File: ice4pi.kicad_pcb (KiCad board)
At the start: 4 copper layers, 65 x 30 mm, 66 parts, among them J1 Pmod 2x6, J2 Raspberry_Pi_2_3, U1 ICE40HX1K-TQ144, U2 N25Q032A13ESC40F, U3 LT3030, U4 DSC1001DI1-012.0000, U5 TFDU4101-TR3

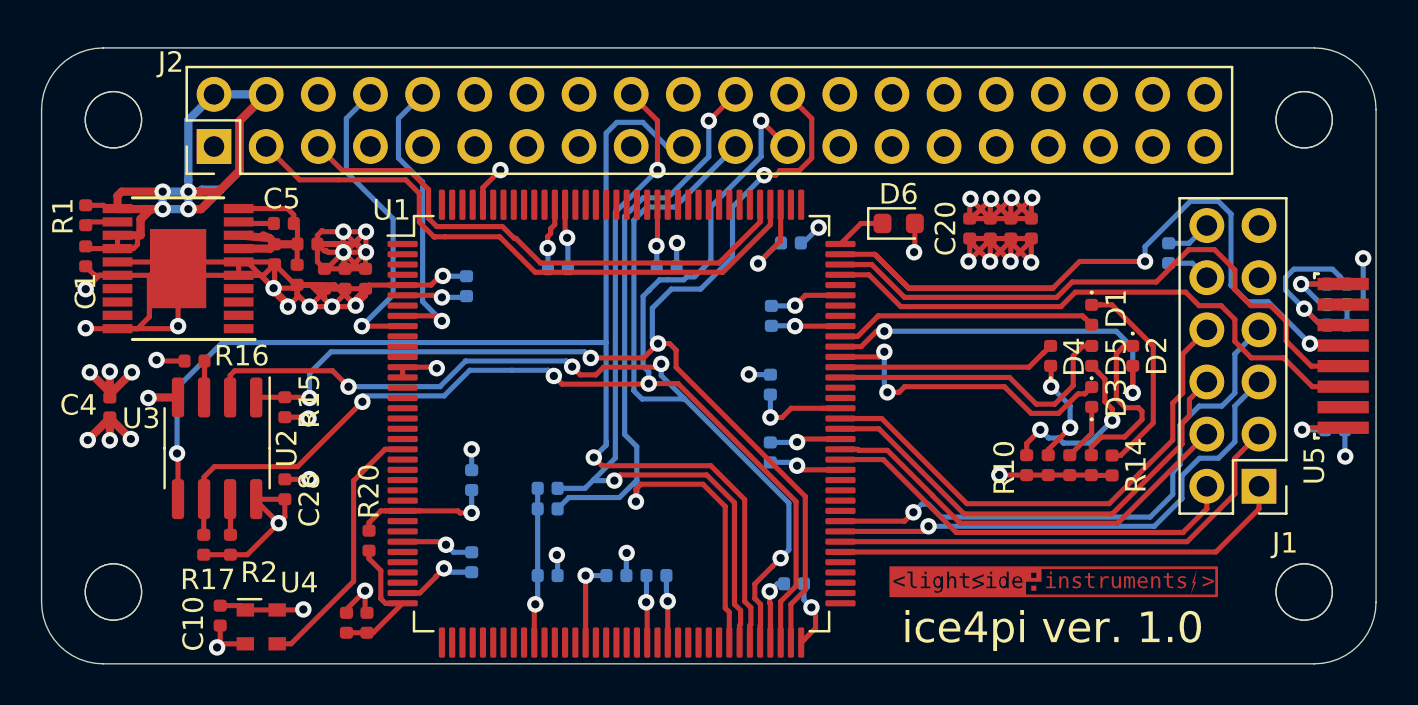
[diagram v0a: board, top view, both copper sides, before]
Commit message: Release ice4pi-1.1
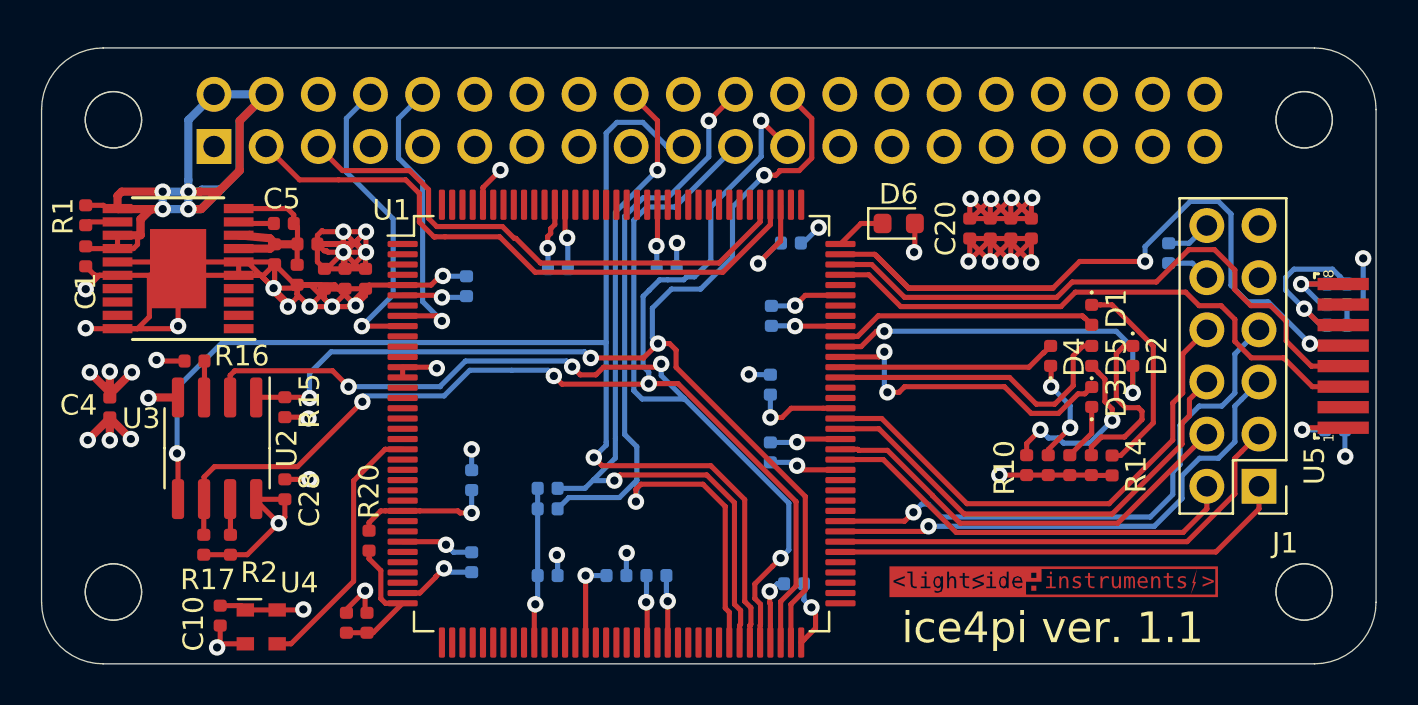
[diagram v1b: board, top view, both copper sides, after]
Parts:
- J2: footprint Connector_PinHeader_2.54mm:PinHeader_2x20_P2.54mm_Vertical -> ice4pi:PinSocket_2x20_P2.54mm_Vertical_1_04mm; moved to B.Cu
- U2: value N25Q032A13ESC40F -> W25Q32JVSSIQ(SOIC-8_208mil)
- turned J2 to 270 degrees
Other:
- board text added: "ice4pi ver. 1.1"
- board text removed: "ice4pi ver. 1.0"
